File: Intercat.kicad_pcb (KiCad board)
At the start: 2 copper layers, 80 x 38 mm, 83 parts, among them J3 DE9_Receptacle, J4 USB_C_Receptacle_USB2.0, T1 LM-NP-1001-B1L, T4 LM-NP-1001-B1L, U1 CP2615-xx-xM, U10 MAX3250, U11 EL357N(C)(TA)-G, U12 EL357N(C)(TA)-G, U2 USBLC6-2SC6, U3 PCM3060, U4 MCP6002, U6 MCP6002, U8 EL357N(C)(TA)-G, U9 EL357N(C)(TA)-G

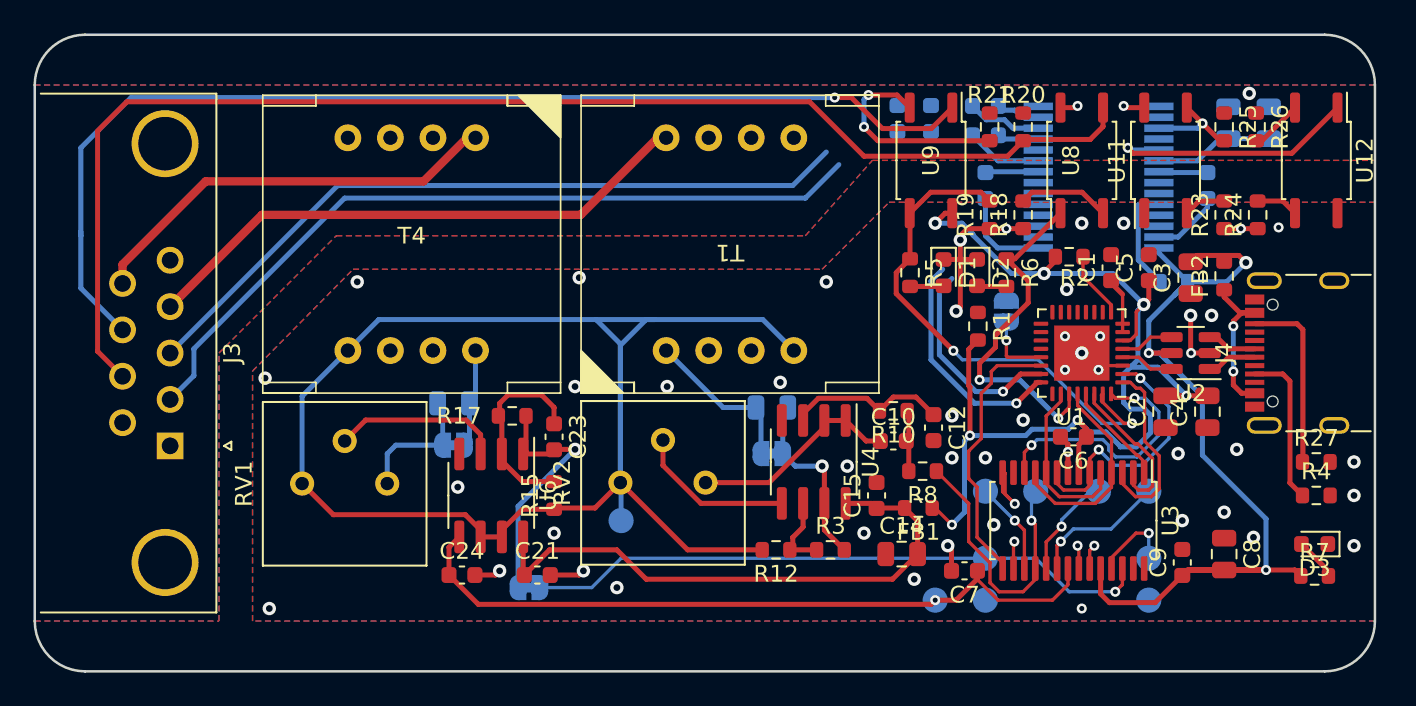
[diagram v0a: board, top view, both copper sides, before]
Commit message: first PCB version
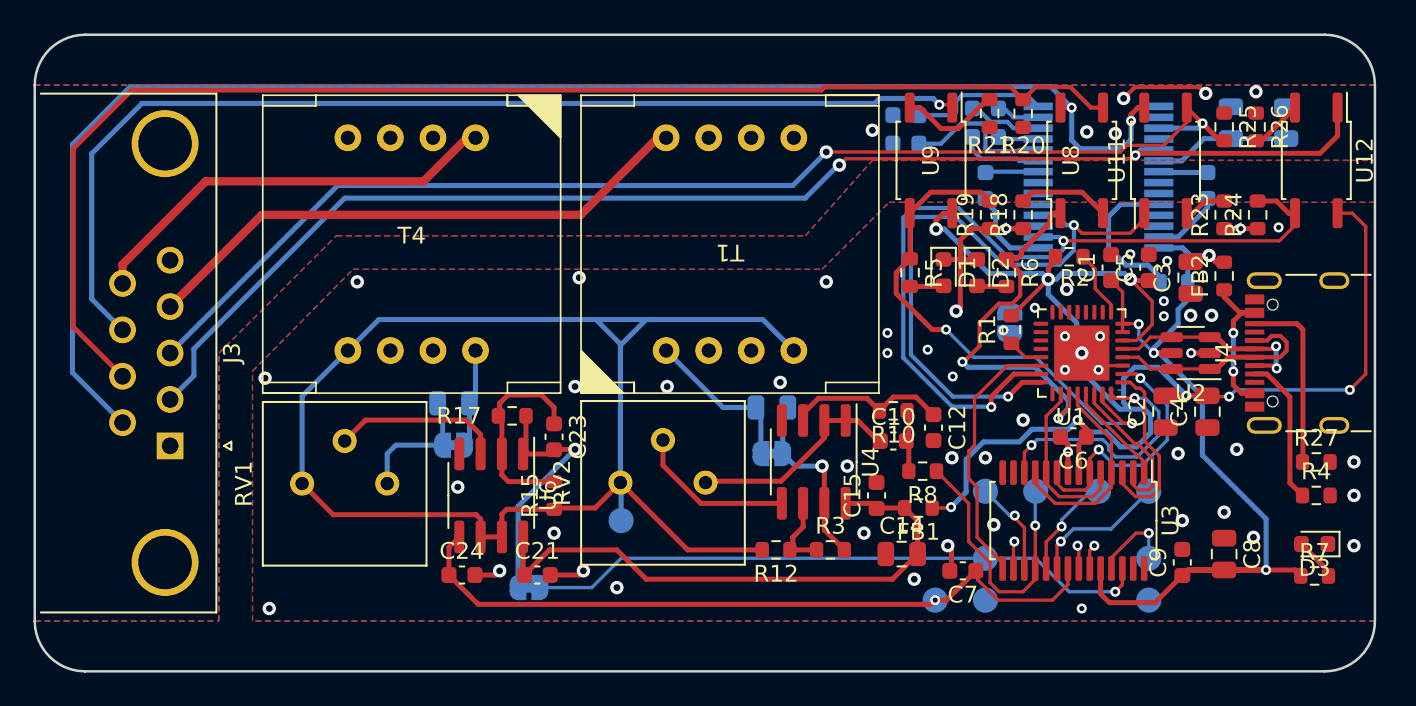
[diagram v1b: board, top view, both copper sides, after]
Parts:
- moved R1 2.01 mm to (158.3, 79.6), turned to 90 degrees
- moved C28 1.58 mm to (152.0, 68.5), turned to 180 degrees
- moved C29 1.51 mm to (152.0, 66.8), turned to 180 degrees
- moved C32 1.04 mm to (174.7, 67.2)
- moved R20 0.80 mm to (159.0, 66.7), turned to 90 degrees
- moved R21 0.80 mm to (157.0, 66.7), turned to 90 degrees
- moved JP1 0.73 mm to (158.2, 79.2)
- moved C27 0.15 mm to (171.4, 67.2)
- moved C31 0.15 mm to (156.8, 66.4)
- moved C30 0.10 mm to (156.8, 68.1)
- moved C7 0.10 mm to (155.4, 94.0)
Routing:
- net VS: track 2.33 -> 88.5 mm
- net /RX: track 14.8 -> 49.7 mm, vias 1 -> 2
- net /TX: track 13.8 -> 37.5 mm, vias 1 -> 2
- net /TX_ISO: track 49.9 -> 73.0 mm, vias 1 -> 2
- net VDD: track 68.3 -> 89.9 mm, vias 7 -> 8
- net /RX_ISO: track 62.3 -> 80.3 mm, vias 1 -> 2
- net Net-(U10-V+): track 0.00 -> 9.09 mm
- net Net-(U10-V-): track 0.00 -> 8.28 mm
- net /D+: track 6.19 -> 13.2 mm
- net Net-(R21-Pad2): track 12.6 -> 6.00 mm, vias 2 -> 0
- net /D-: track 6.19 -> 12.5 mm, vias 0 -> 2
- net GNDA: track 0.00 -> 5.69 mm, vias 1 -> 6
- net unconnected-(U3-ZEROL-Pad14): track 4.04 -> 0.00 mm, vias 1 -> 0
- net Net-(U10-nSHDN): track 6.36 -> 9.25 mm
- net /RTS: track 20.9 -> 23.4 mm
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- added copper zone on B.Cu, net VDD
